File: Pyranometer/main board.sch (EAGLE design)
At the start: 9 parts

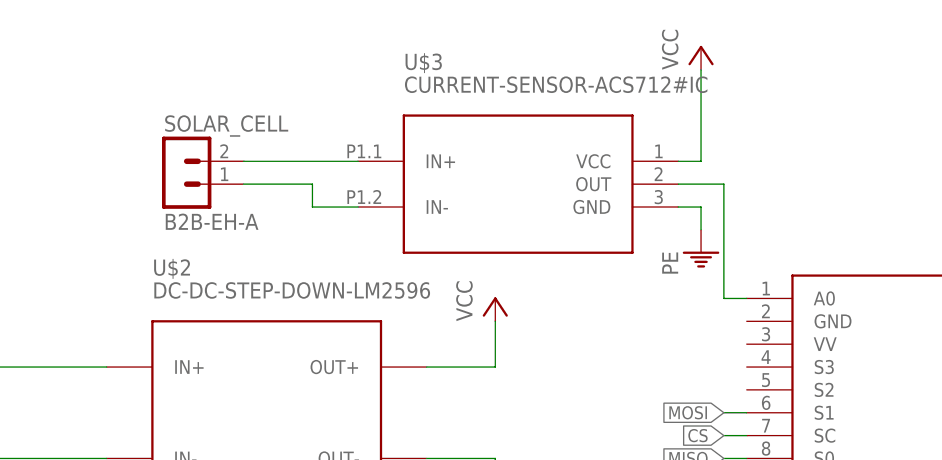
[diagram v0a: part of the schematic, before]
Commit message: backup
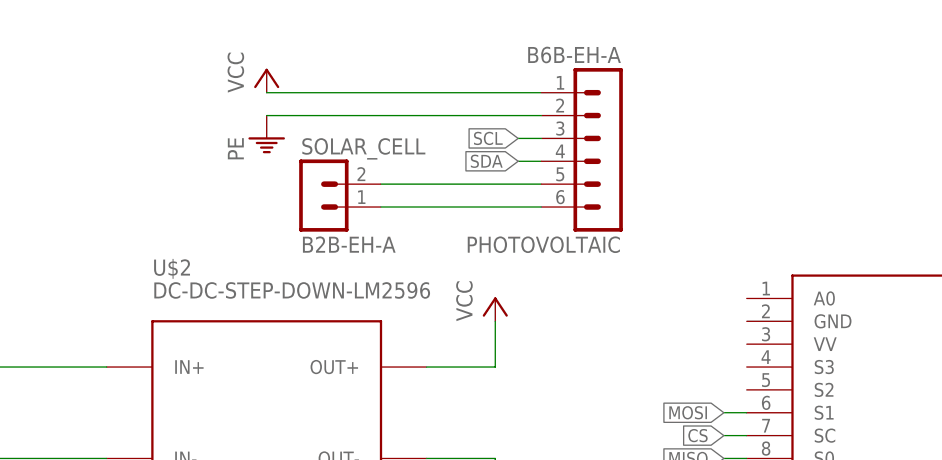
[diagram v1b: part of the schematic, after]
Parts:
- removed U$3: CURRENT-SENSOR-ACS712#IC, diy-modules:CURRENT-SENSOR-ACS712#IC
- added PHOTOVOLTAIC: B6B-EH-A, con-JST EH:B6B-EH-A
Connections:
- removed net N$6: SOLAR_CELL.1, U$3.IN-
- net N$1: now also PHOTOVOLTAIC.6, SOLAR_CELL.1; no longer U$1.A0, U$3.OUT
- net N$5: now also PHOTOVOLTAIC.5; no longer U$3.IN+
- net PE: now also PHOTOVOLTAIC.2; no longer U$3.GND
- net SCL: now also PHOTOVOLTAIC.3
- net SDA: now also PHOTOVOLTAIC.4
- net VCC: now also PHOTOVOLTAIC.1; no longer U$3.VCC
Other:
- moved on the sheet: SOLAR_CELL
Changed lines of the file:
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@@
 <part name="LCD" library="con-JST EH" deviceset="B4B-EH" device="-A"/>
 <part name="SUPPLY" library="con-JST EH" deviceset="B2B-EH" device="-A"/>
-<part name="U$3" library="diy-modules" deviceset="CURRENT-SENSOR-ACS712#IC" device=""/>
 <part name="SOLAR_CELL" library="con-JST EH" deviceset="B2B-EH" device="-A"/>
 <part name="SWITCH" library="con-JST EH" deviceset="B2B-EH" device="-A"/>
@@
 <part name="P+6" library="supply1" deviceset="VCC" device=""/>
 <part name="PE6" library="supply1" deviceset="PE" device=""/>
+<part name="PHOTOVOLTAIC" library="con-JST EH" deviceset="B6B-EH" device="-A"/>
 </parts>
 <sheets>
@@
 <instance part="LCD" gate="G$1" x="88.9" y="27.94"/>
 <instance part="SUPPLY" gate="G$1" x="-48.26" y="83.82"/>
-<instance part="U$3" gate="G$1" x="20.32" y="83.82"/>
-<instance part="SOLAR_CELL" gate="G$1" x="-17.78" y="86.36"/>
+<instance part="SOLAR_CELL" gate="G$1" x="-2.54" y="83.82"/>
 <instance part="SWITCH" gate="G$1" x="-48.26" y="66.04"/>
-<instance part="P+1" gate="VCC" x="40.64" y="99.06"/>
-<instance part="PE1" gate="M" x="40.64" y="76.2"/>
+<instance part="P+1" gate="VCC" x="-7.62" y="96.52"/>
+<instance part="PE1" gate="M" x="-7.62" y="88.9"/>
 <instance part="PE2" gate="M" x="114.3" y="20.32"/>
 <instance part="PE3" gate="M" x="116.84" y="78.74"/>
@@
 <instance part="P+6" gate="VCC" x="139.7" y="55.88"/>
 <instance part="PE6" gate="M" x="139.7" y="48.26"/>
+<instance part="PHOTOVOLTAIC" gate="G$1" x="30.48" y="86.36" rot="R180"/>
 </instances>
 <busses>
 </busses>
 <nets>
-<net name="N$1" class="0">
-<segment>
-<pinref part="U$1" gate="G$1" pin="A0"/>
-<wire x1="45.72" y1="71.12" x2="43.18" y2="71.12" width="0.1524" layer="91"/>
-<wire x1="43.18" y1="71.12" x2="43.18" y2="83.82" width="0.1524" layer="91"/>
-<pinref part="U$3" gate="G$1" pin="OUT"/>
-<wire x1="43.18" y1="83.82" x2="38.1" y2="83.82" width="0.1524" layer="91"/>
-</segment>
-</net>
 <net name="N$2" class="0">
 <segment>
@@
 </segment>
 <segment>
-<pinref part="U$3" gate="G$1" pin="VCC"/>
-<pinref part="P+1" gate="VCC" pin="VCC"/>
-<wire x1="38.1" y1="86.36" x2="40.64" y2="86.36" width="0.1524" layer="91"/>
-<wire x1="40.64" y1="86.36" x2="40.64" y2="96.52" width="0.1524" layer="91"/>
-</segment>
-<segment>
 <pinref part="U$1" gate="G$1" pin="VIN"/>
 <pinref part="P+5" gate="VCC" pin="VCC"/>
@@
 <wire x1="139.7" y1="53.34" x2="124.46" y2="53.34" width="0.1524" layer="91"/>
 </segment>
+<segment>
+<pinref part="PHOTOVOLTAIC" gate="G$1" pin="1"/>
+<pinref part="P+1" gate="VCC" pin="VCC"/>
+<wire x1="-7.62" y1="93.98" x2="22.86" y2="93.98" width="0.1524" layer="91"/>
+</segment>
 </net>
 <net name="PE" class="0">
@@
 </segment>
 <segment>
-<pinref part="PE1" gate="M" pin="PE"/>
-<wire x1="40.64" y1="78.74" x2="40.64" y2="81.28" width="0.1524" layer="91"/>
-<pinref part="U$3" gate="G$1" pin="GND"/>
-<wire x1="40.64" y1="81.28" x2="38.1" y2="81.28" width="0.1524" layer="91"/>
-</segment>
-<segment>
 <pinref part="U$1" gate="G$1" pin="GND@1"/>
 <pinref part="PE4" gate="M" pin="PE"/>
@@
 <wire x1="139.7" y1="50.8" x2="124.46" y2="50.8" width="0.1524" layer="91"/>
 </segment>
-</net>
-<net name="N$5" class="0">
-<segment>
-<pinref part="U$3" gate="G$1" pin="IN+"/>
-<pinref part="SOLAR_CELL" gate="G$1" pin="2"/>
-<wire x1="-10.16" y1="86.36" x2="2.54" y2="86.36" width="0.1524" layer="91"/>
-</segment>
-</net>
-<net name="N$6" class="0">
-<segment>
-<pinref part="SOLAR_CELL" gate="G$1" pin="1"/>
-<wire x1="-10.16" y1="83.82" x2="-2.54" y2="83.82" width="0.1524" layer="91"/>
-<wire x1="-2.54" y1="83.82" x2="-2.54" y2="81.28" width="0.1524" layer="91"/>
-<pinref part="U$3" gate="G$1" pin="IN-"/>
-<wire x1="-2.54" y1="81.28" x2="2.54" y2="81.28" width="0.1524" layer="91"/>
+<segment>
+<pinref part="PHOTOVOLTAIC" gate="G$1" pin="2"/>
+<pinref part="PE1" gate="M" pin="PE"/>
+<wire x1="-7.62" y1="91.44" x2="22.86" y2="91.44" width="0.1524" layer="91"/>
 </segment>
 </net>
@@
 <wire x1="99.06" y1="30.48" x2="96.52" y2="30.48" width="0.1524" layer="91"/>
 </segment>
+<segment>
+<pinref part="PHOTOVOLTAIC" gate="G$1" pin="3"/>
+<wire x1="22.86" y1="88.9" x2="20.32" y2="88.9" width="0.1524" layer="91"/>
+<label x="20.32" y="88.9" size="1.4224" layer="95" rot="R180" xref="yes"/>
+</segment>
 </net>
 <net name="SDA" class="0">
@@
 <wire x1="96.52" y1="27.94" x2="99.06" y2="27.94" width="0.1524" layer="91"/>
 </segment>
+<segment>
+<pinref part="PHOTOVOLTAIC" gate="G$1" pin="4"/>
+<wire x1="22.86" y1="86.36" x2="20.32" y2="86.36" width="0.1524" layer="91"/>
+<label x="20.32" y="86.36" size="1.4224" layer="95" rot="R180" xref="yes"/>
+</segment>
 </net>
 <net name="CS" class="0">
@@
 </segment>
 </net>
+<net name="N$1" class="0">
+<segment>
+<pinref part="PHOTOVOLTAIC" gate="G$1" pin="6"/>
+<pinref part="SOLAR_CELL" gate="G$1" pin="1"/>
+<wire x1="5.08" y1="81.28" x2="22.86" y2="81.28" width="0.1524" layer="91"/>
+</segment>
+</net>
+<net name="N$5" class="0">
+<segment>
+<pinref part="PHOTOVOLTAIC" gate="G$1" pin="5"/>
+<pinref part="SOLAR_CELL" gate="G$1" pin="2"/>
+<wire x1="5.08" y1="83.82" x2="22.86" y2="83.82" width="0.1524" layer="91"/>
+</segment>
+</net>
